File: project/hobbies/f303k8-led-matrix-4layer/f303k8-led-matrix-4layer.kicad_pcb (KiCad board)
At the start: 4 copper layers, 40 x 20 mm, 103 parts, among them J1 USB_C_Receptacle_USB2.0_16P, J2 Boot, U1 USBLC6-2SC6, U2 CH552E, U3 CH213K, U4 STM32F303K8Tx, U5 NJM12888

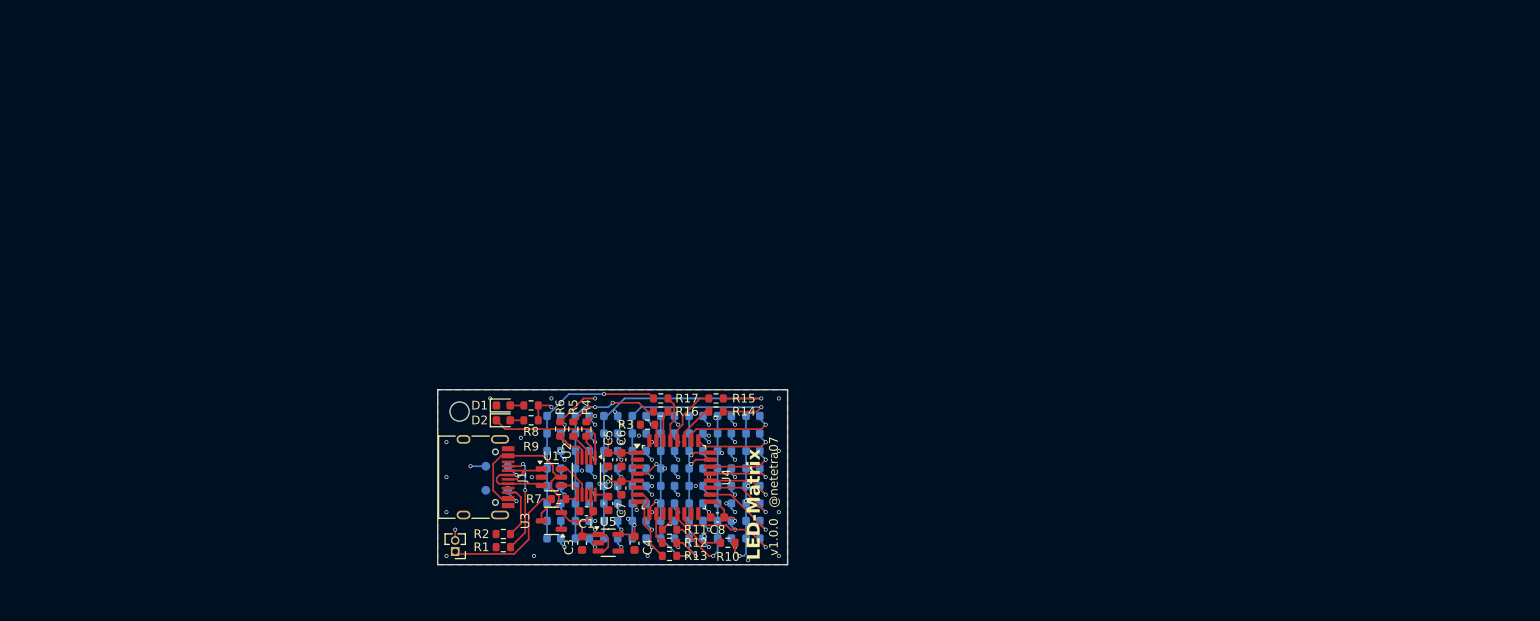
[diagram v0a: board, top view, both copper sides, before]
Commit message: 2026/01/30/13:22
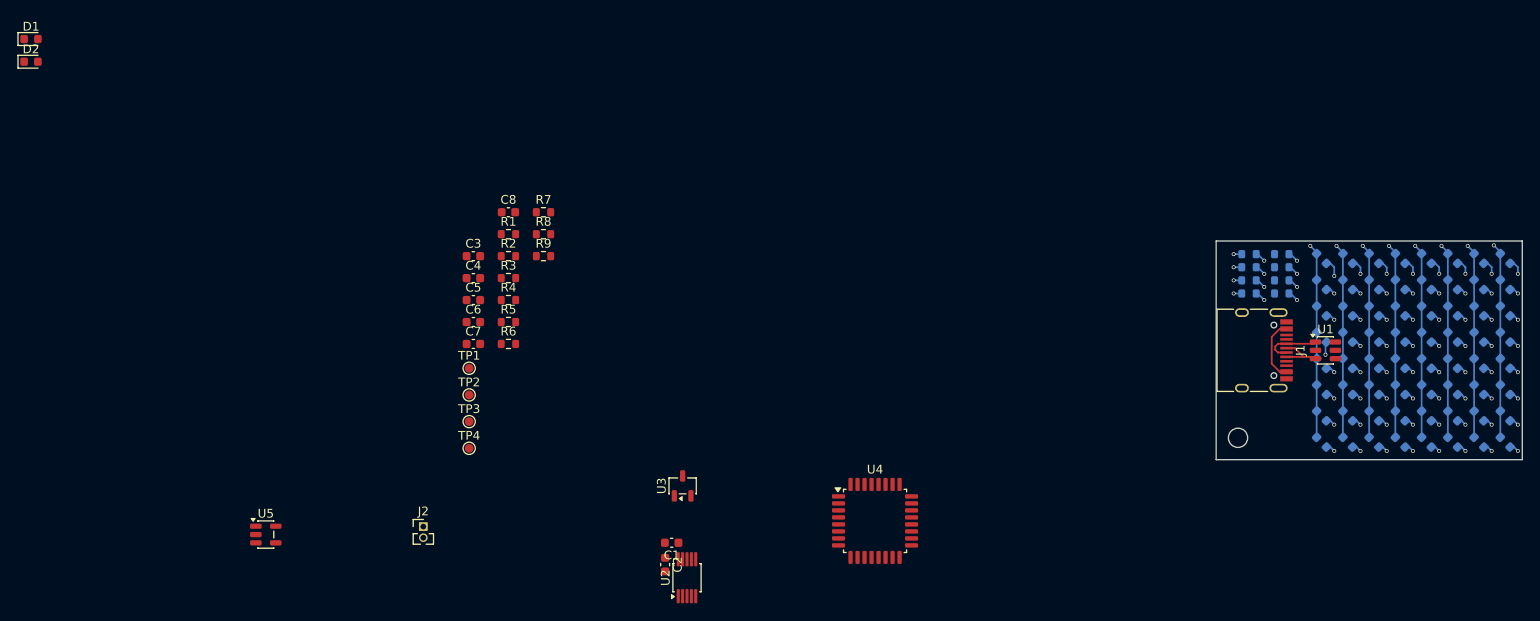
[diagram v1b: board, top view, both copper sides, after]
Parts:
- R10, R11, R12, R13, R14, R15, R16, R17: moved to B.Cu
- TP1, TP2, TP3, TP4: moved to F.Cu
- moved D59 105.6 mm to (222.0, 91.0), turned to 135 degrees
- moved D60 102.7 mm to (219.0, 91.0), turned to 135 degrees
- moved D11 100.1 mm to (222.0, 73.0), turned to 135 degrees
- moved D61 99.9 mm to (216.0, 91.0), turned to 135 degrees
- moved D27 99.9 mm to (222.0, 79.0), turned to 135 degrees
- moved D51 99.3 mm to (222.0, 88.0), turned to 135 degrees
- moved D12 97.5 mm to (219.0, 73.0), turned to 135 degrees
- moved D13 97.4 mm to (216.0, 73.0), turned to 135 degrees
- moved D28 97.2 mm to (219.0, 79.0), turned to 135 degrees
- moved D62 97.1 mm to (213.0, 91.0), turned to 135 degrees
- moved D29 97.1 mm to (216.0, 79.0), turned to 135 degrees
- moved D63 96.9 mm to (210.0, 91.0), turned to 135 degrees
- moved D52 96.5 mm to (219.0, 88.0), turned to 135 degrees
- moved D14 94.8 mm to (213.0, 73.0), turned to 135 degrees
- moved D15 94.7 mm to (210.0, 73.0), turned to 135 degrees
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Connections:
- D10 pad 1: ROW_B -> ROW_A
- D11 pad 1: ROW_A -> ROW_B
- D12 pad 2: Net-(D11-A) -> Net-(D12-A)
- D13 pad 1: ROW_A -> ROW_B
- D14 pad 2: Net-(D13-A) -> Net-(D14-A)
- D15 pad 1: ROW_A -> ROW_B
- D16 pad 2: Net-(D15-A) -> Net-(D16-A)
- D17 pad 1: ROW_A -> ROW_B
- D18 pad 2: Net-(D17-A) -> Net-(D10-A)
- D19 pad 2: Net-(D19-A) -> Net-(D11-A)
- D20 pad 1: ROW_D -> ROW_C
- D20 pad 2: Net-(D19-A) -> Net-(D12-A)
- D21 pad 2: Net-(D21-A) -> Net-(D13-A)
- D22 pad 1: ROW_D -> ROW_C
- D22 pad 2: Net-(D21-A) -> Net-(D14-A)
- D23 pad 2: Net-(D23-A) -> Net-(D15-A)
- D24 pad 1: ROW_D -> ROW_C
- D24 pad 2: Net-(D23-A) -> Net-(D16-A)
- D25 pad 2: Net-(D10-A) -> Net-(D17-A)
- D26 pad 1: ROW_D -> ROW_C
- D27 pad 1: ROW_C -> ROW_D
- D28 pad 2: Net-(D11-A) -> Net-(D12-A)
- D29 pad 1: ROW_C -> ROW_D
- D3 pad 2: Net-(D19-A) -> Net-(D11-A)
- D30 pad 2: Net-(D13-A) -> Net-(D14-A)
- D31 pad 1: ROW_C -> ROW_D
- D32 pad 2: Net-(D15-A) -> Net-(D16-A)
- D33 pad 1: ROW_C -> ROW_D
- D34 pad 2: Net-(D17-A) -> Net-(D10-A)
- D35 pad 2: Net-(D19-A) -> Net-(D11-A)
- D36 pad 1: ROW_F -> ROW_E
- D36 pad 2: Net-(D19-A) -> Net-(D12-A)
- D37 pad 1: ROW_G -> ROW_E
- D37 pad 2: Net-(D19-A) -> Net-(D13-A)
- D38 pad 1: ROW_H -> ROW_E
- D38 pad 2: Net-(D19-A) -> Net-(D14-A)
- D39 pad 2: Net-(D21-A) -> Net-(D15-A)
- D4 pad 1: ROW_B -> ROW_A
- D4 pad 2: Net-(D19-A) -> Net-(D12-A)
- D40 pad 1: ROW_F -> ROW_E
- D40 pad 2: Net-(D21-A) -> Net-(D16-A)
- D41 pad 1: ROW_G -> ROW_E
- D41 pad 2: Net-(D21-A) -> Net-(D17-A)
- D42 pad 1: ROW_H -> ROW_E
- D42 pad 2: Net-(D21-A) -> Net-(D10-A)
- D43 pad 1: ROW_E -> ROW_F
- D43 pad 2: Net-(D23-A) -> Net-(D11-A)
- D44 pad 2: Net-(D23-A) -> Net-(D12-A)
- D45 pad 1: ROW_G -> ROW_F
- D45 pad 2: Net-(D23-A) -> Net-(D13-A)
- D46 pad 1: ROW_H -> ROW_F
- D46 pad 2: Net-(D23-A) -> Net-(D14-A)
- D47 pad 1: ROW_E -> ROW_F
- D47 pad 2: Net-(D10-A) -> Net-(D15-A)
- D48 pad 2: Net-(D10-A) -> Net-(D16-A)
- D49 pad 1: ROW_G -> ROW_F
- D49 pad 2: Net-(D10-A) -> Net-(D17-A)
- D5 pad 2: Net-(D21-A) -> Net-(D13-A)
- D50 pad 1: ROW_H -> ROW_F
- D51 pad 1: ROW_E -> ROW_G
- D52 pad 1: ROW_F -> ROW_G
- D52 pad 2: Net-(D11-A) -> Net-(D12-A)
- D53 pad 2: Net-(D11-A) -> Net-(D13-A)
- D54 pad 1: ROW_H -> ROW_G
- D54 pad 2: Net-(D11-A) -> Net-(D14-A)
- D55 pad 1: ROW_E -> ROW_G
- D55 pad 2: Net-(D13-A) -> Net-(D15-A)
- D56 pad 1: ROW_F -> ROW_G
- D56 pad 2: Net-(D13-A) -> Net-(D16-A)
- D57 pad 2: Net-(D13-A) -> Net-(D17-A)
- D58 pad 1: ROW_H -> ROW_G
- D58 pad 2: Net-(D13-A) -> Net-(D10-A)
- D59 pad 1: ROW_E -> ROW_H
- D59 pad 2: Net-(D15-A) -> Net-(D11-A)
- D6 pad 1: ROW_B -> ROW_A
- D6 pad 2: Net-(D21-A) -> Net-(D14-A)
- D60 pad 1: ROW_F -> ROW_H
- D60 pad 2: Net-(D15-A) -> Net-(D12-A)
- D61 pad 1: ROW_G -> ROW_H
- D61 pad 2: Net-(D15-A) -> Net-(D13-A)
- D62 pad 2: Net-(D15-A) -> Net-(D14-A)
- D63 pad 1: ROW_E -> ROW_H
- D63 pad 2: Net-(D17-A) -> Net-(D15-A)
- D64 pad 1: ROW_F -> ROW_H
- D64 pad 2: Net-(D17-A) -> Net-(D16-A)
- D65 pad 1: ROW_G -> ROW_H
- D66 pad 2: Net-(D17-A) -> Net-(D10-A)
- D7 pad 2: Net-(D23-A) -> Net-(D15-A)
- D8 pad 1: ROW_B -> ROW_A
- D8 pad 2: Net-(D23-A) -> Net-(D16-A)
- D9 pad 2: Net-(D10-A) -> Net-(D17-A)
- R10 pad 2: Net-(D19-A) -> Net-(D11-A)
- R11 pad 2: Net-(D21-A) -> Net-(D12-A)
- R12 pad 2: Net-(D23-A) -> Net-(D13-A)
- R13 pad 2: Net-(D10-A) -> Net-(D14-A)
- R14 pad 2: Net-(D11-A) -> Net-(D15-A)
- R15 pad 2: Net-(D13-A) -> Net-(D16-A)
- R16 pad 2: Net-(D15-A) -> Net-(D17-A)
- R17 pad 2: Net-(D17-A) -> Net-(D10-A)
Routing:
- net Net-(D12-A): track 0.00 -> 45.2 mm, vias 0 -> 2
- net Net-(D16-A): track 0.00 -> 38.6 mm, vias 0 -> 2
- net Net-(D14-A): track 0.00 -> 38.0 mm, vias 0 -> 2
- net +3.3V: track 22.2 -> 0.00 mm, vias 7 -> 0
- net Net-(D21-A): track 21.6 -> 0.00 mm, vias 1 -> 0
- net SWCLK: track 21.6 -> 0.00 mm, vias 2 -> 0
- net RX: track 21.4 -> 0.00 mm, vias 2 -> 0
- net SWDIO: track 19.5 -> 0.00 mm, vias 2 -> 0
- net Net-(D23-A): track 19.1 -> 0.00 mm, vias 1 -> 0
- net Net-(D15-A): track 24.0 -> 42.8 mm, vias 1 -> 2
- net Net-(D19-A): track 18.3 -> 0.00 mm, vias 1 -> 0
- net TX: track 16.8 -> 0.00 mm, vias 2 -> 0
- net Net-(D11-A): track 33.7 -> 49.4 mm, vias 1 -> 2
- net Net-(J2-Pin_1): track 15.5 -> 0.00 mm
- net Net-(U1-VBUS): track 22.2 -> 7.22 mm
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- removed copper zone on In1.Cu, net +3.3V
- removed copper zone on B.Cu, net GND
- removed copper zone on F.Cu, net GND
- removed copper zone on In2.Cu, net GND
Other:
- board size 40 x 20 mm -> 35 x 25 mm
- board text removed: "3V3"
- board text removed: "@netetra07"
- board text removed: "GND"
- board text removed: "LED-Matrix"
- board text removed: "RX"
- board text removed: "TX"
- board text removed: "v1.0.0"
